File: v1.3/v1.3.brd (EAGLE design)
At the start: 100 x 50.2 mm, 88 parts, among them IC1 LM1117-33, IC2 ENC28J60, K2 G5V1, K3 JRC-21F(4100), T1 2N2222, T2 2N2222, T3 2N2222, T4 2N2222, U1 ATMEGA328P, X1 32.768kHz, X10 22-23-2031, X12 12MHZ, X2 16MHz, X3 25MHz, X9 22-23-2031

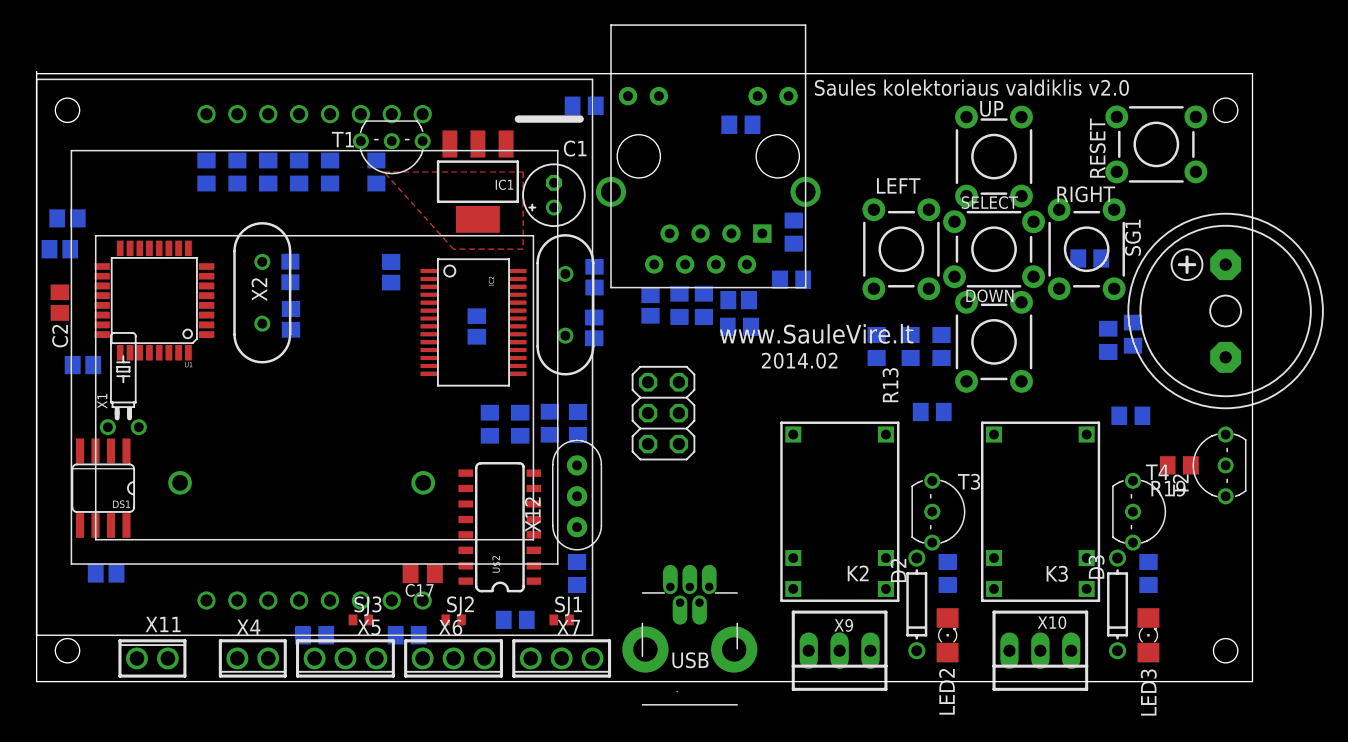
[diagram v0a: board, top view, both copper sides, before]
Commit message: 1.3 versija
programa su 3 klavisais
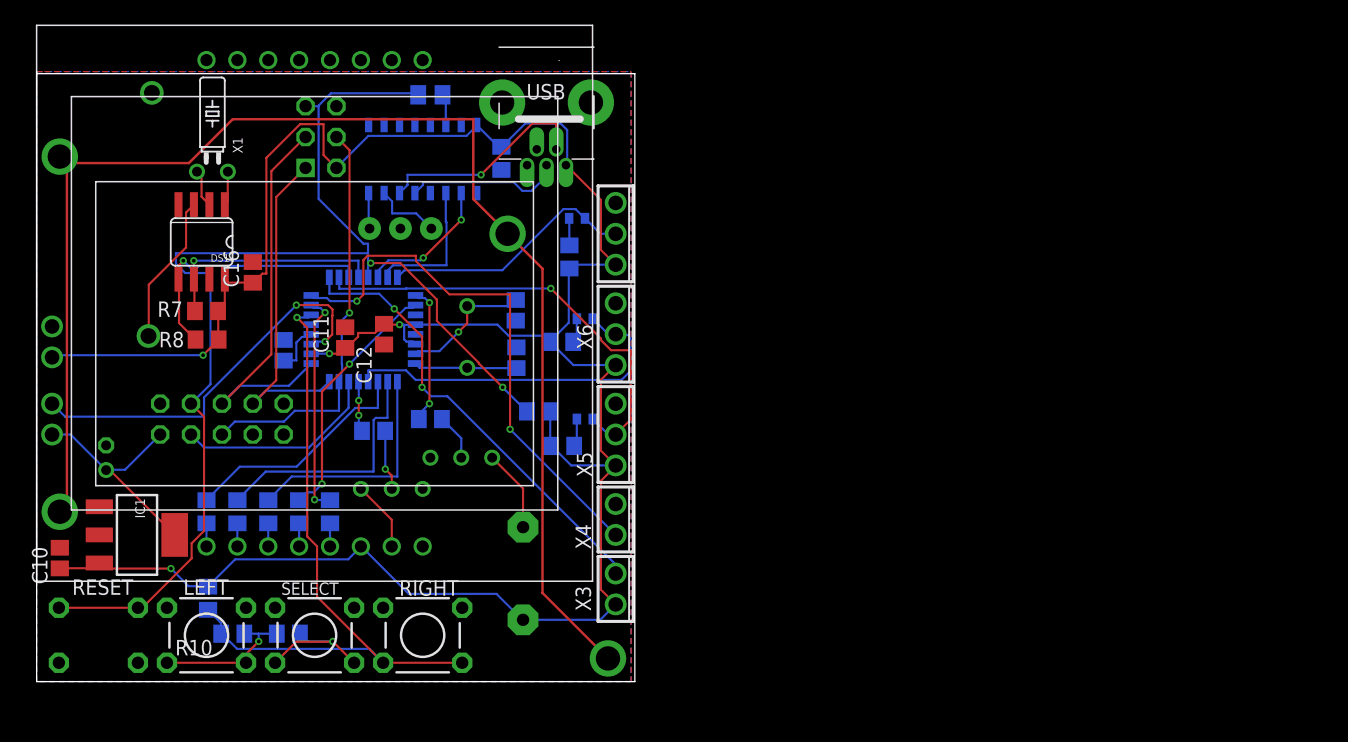
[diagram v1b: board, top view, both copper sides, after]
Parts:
- removed C13: 0.1u, rcl:C0805
- removed C14: 100n, resistor:C0805
- removed C4, C5: 0.1µ, resistor:C0805
- removed C6, C7: 18p, resistor:C0805
- removed CAP: 10u, resistor:C0805
- removed D2, D3: (no value), adafruit:DO-1N4148
- removed DOWN, UP: (no value), SparkFun-Electromechanical:TACTILE-PTH
- removed IC2: ENC28J60, SparkFun-DigitalIC:SSOP28DB
- removed K2: G5V1, relay:G5V1
- removed K3: JRC-21F(4100), relay:G5V1
- removed L1: Bead, rcl:R0805
- removed LED2, LED3: (no value), adafruit:1206
- removed R15, R16, R20: 49, rcl:R0805
- removed R17, R22, R23, R24, R25, R26: 10k, rcl:R0805
- removed R18: 4k7, rcl:R0805
- removed R21: 1k, rcl:R0805
- removed RBS: 2.32K, rcl:R0805
- removed REA, REB: 330, rcl:R0805
- removed RJ1: HR911105A, CONNECTER:HR911105A
- removed T3, T4: 2N2222, adafruit:TO92-EBC-OVAL
- removed X10, X9: 22-23-2031, con-molex:22-23-2031
- removed X12: 12MHZ, adafruit:CERM_OSC
- added ENC28J60: (no value), pinhead:2X05
- added R116: 10k, rcl:R0805
- added X8: (no value), con-phoenix-254:2POL254
- added Y1: 12mhz, SparkFun-FreqCtrl:RESONATOR-PTH
- BAT1, LEFT, RIGHT, SELECT, USB, X11, X4, X5, X6, X7: value (none) -> (none)
- C17: value (none) -> 0.1uF
- ISP: value (none) -> isp
- R1, R3: value 470 -> 10k
- R10: value 330 -> 2k
- R12: value 620 -> 4k7
- R13: value 1k -> 4k7
- R14: value 49 -> 4k7
- R2, R4: value 3k3 -> 10k
- R5: value 4k7 -> 10k
- R6: value 4k7 -> 1k
- SJ1, SJ2, SJ3: value 0R -> (none)
- X3: value 25MHz -> (none); device SparkFun:HC49US -> con-phoenix-254:2POL254
- moved RESET 95.9 mm to (5.08, 3.81), flipped to the bottom, turned to 180 degrees
- moved R1 77.6 mm to (14.0, 14.0), turned to 270 degrees
- moved R9 77.0 mm to (14.1, 6.86), turned to 90 degrees
- moved R10 76.9 mm to (16.1, 3.94), turned to 0 degrees
- moved R2 73.9 mm to (16.5, 14.0), turned to 270 degrees
- moved LEFT 65.4 mm to (14.0, 3.81), turned to 0 degrees
- moved SELECT 64.3 mm to (22.9, 3.81)
- moved RIGHT 63.2 mm to (31.8, 3.81), turned to 0 degrees
- moved R19 61.7 mm to (32.4, 21.6), flipped to the bottom, turned to 0 degrees
- moved SG1 61.7 mm to (40.0, 8.89), flipped to the bottom, turned to 270 degrees
- moved T2 61.6 mm to (34.9, 17.1), flipped to the bottom, turned to 180 degrees
- moved R11 58.7 mm to (20.7, 3.94), turned to 0 degrees
- moved R3 56.1 mm to (19.1, 14.0), turned to 270 degrees
- moved USB 55.4 mm to (41.9, 52.2), turned to 180 degrees
- moved R4 52.7 mm to (21.6, 14.0), turned to 270 degrees
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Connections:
- net N$35 renamed AREF
- net TXD renamed D1/TXD
- removed net D11: IC2.7, ISP.4, U1.15
- removed net D12: IC2.6, ISP.1, U1.16
- removed net D13: IC2.8, U1.17
- removed net LEDA: REA.2, RJ1.G+
- removed net LEDB: REB.2, RJ1.Y+
- removed net N$12: D3.A, K3.9, R1.2, T4.C
- removed net N$13: R2.1, T4.B
- removed net N$14: K2.1, X9.1
- removed net N$16: K3.10, X10.2
- removed net N$19: K3.5, K3.6, X10.3
- removed net N$20: K3.1, X10.1
- removed net N$21: LED3.C, R1.1
- removed net N$22: R22.1, U$1.P$5
- removed net N$23: R25.1, U$1.P$2
- removed net N$24: R24.1, U$1.P$3
- removed net N$25: R23.1, U$1.P$4
- removed net N$34: IC2.27, REA.1
- removed net N$37: IC2.26, REB.1
- removed net N$38: U$2.8, X12.P$3
- removed net N$39: CAP.1, IC2.1
- removed net N$41: C6.1, IC2.24, X3.2
- removed net N$42: C7.1, IC2.23, X3.1
- removed net N$46: R17.1, RESET.3, RESET.4, U1.29
- removed net N$54: C5.2, R15.1, R16.2
- removed net N$59: IC2.14, RBS.2
- removed net N$7 (its old number): LED2.C, R3.1
- removed net N$9: R10.1, R12.2, UP.3, UP.4
- removed net RD+: IC2.13, R15.2, RJ1.RD+
- removed net RD-: IC2.12, R16.1, RJ1.RD-
- removed net RXD: U1.30
- removed net SCK: ISP.3
- removed net SCL: DS1.6, R7.1, U1.28, X4.1
- removed net SDA: DS1.5, R8.1, U1.27, X4.2
- removed net TCT: C4.2, L1.1, R14.2, R20.1, RJ1.P4
- removed net TD+: IC2.17, R20.2, RJ1.TD+
- removed net TD-: IC2.16, R14.1, RJ1.TD-
- removed net V$: R26.1, U$1.P$1
- removed net VIN: ISP.2
- new net A4/SDA: DS1.5, R8.1, U1.27
- new net A5/SCL: DS1.6, R7.1, U1.28
- new net D0/RXD: U$2.2, U1.30
- new net D11/MOSI: ENC28J60.5, ISP.4, U1.15
- new net D12/MISO: ENC28J60.4, ISP.1, U1.16
- new net D13/SCK: ENC28J60.6, ISP.3, U1.17
- net +3V3: now also ENC28J60.9, X8.2; no longer C14.1, IC2.15, IC2.19, IC2.20, IC2.25, IC2.28
- net +5V: now also ISP.2, R116.2, R12.1, R13.1, R14.1, U$1.P$14, X3.2; no longer D2.C, D3.C, K2.2, K3.2, L1.2, LED2.A, LED3.A, R17.2, R18.1, R5.1, R6.1, U$1.P$6
- net A0: now also R5.1; no longer SJ3.2, X5.2
- net A1: now also X4.2; no longer SJ2.2, X6.2
- net A2: now also X3.1; no longer R2.2
- net A3: now also SJ3.2, X5.2; no longer R4.2
- net A6: now also X8.1; no longer R10.2, R9.1, RIGHT.3, RIGHT.4
- net A7: now also R10.2, R9.1, RIGHT.3, RIGHT.4
- net D10: now also ENC28J60.7; no longer R21.2
- net D3: now also R19.2; no longer R22.2
- net D4: now also R4.1; no longer R23.2
- net D5: now also R3.1; no longer R24.2
- net D6: now also R2.1; no longer R25.2
- net D7: now also R1.1; no longer R26.2
- net D8: now also SJ2.2, X6.2; no longer IC2.9
- net D9: now also R6.2; no longer R19.2
- net GND: now also ENC28J60.10, U$1.P$16, X4.1, Y1.2; no longer C13.1, C14.2, C4.1, C5.1, C6.2, C7.2, CAP.2, DOWN.1, DOWN.2, IC2.11, IC2.18, IC2.2, IC2.21, IC2.22, RBS.1, RJ1.G-, RJ1.GND, RJ1.SHIELD0, RJ1.SHIELD1, RJ1.Y-, T3.E, T4.E, U$1.P$8, UP.1, UP.2, X12.P$2
- net N$1: now also R10.1; no longer R13.1
- net N$10: now also Y1.1; no longer X12.P$1
- net N$17: now also R13.2; no longer R6.2
- net N$2: now also R5.2, U$1.P$13; no longer D2.A, K2.9, R3.2, T3.C
- net N$26: now also U$1.P$15; no longer U$1.P$7
- net N$28: now also R14.2; no longer R18.2
- net N$3: now also R4.2, U$1.P$12; no longer R4.1, T3.B
- net N$31: now also R12.2; no longer R5.2
- net N$4: now also R3.2, U$1.P$11; no longer K2.5, K2.6, X9.3
- net N$40: now also U$2.8, Y1.3; no longer C13.2, U$2.4
- net N$44: now also R6.1; no longer R21.1
- net N$5: now also R2.2, U$1.P$10; no longer K2.10, X9.2
- net N$6: now also R1.2, U$1.P$9; no longer DOWN.3, DOWN.4, R12.1, R13.2
- net RESET: now also ENC28J60.8, R116.1, RESET.3, RESET.4, U1.29; no longer IC2.10
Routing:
- net +5V: track 0.00 -> 201.9 mm, vias 0 -> 4
- net GND: track 0.00 -> 114.4 mm, vias 0 -> 4
- net RESET: track 0.00 -> 102.4 mm, vias 0 -> 2
- net A7: track 0.00 -> 55.8 mm, vias 0 -> 1
- net A1: track 0.00 -> 44.7 mm, vias 0 -> 2
- net A2: track 0.00 -> 37.3 mm, vias 0 -> 2
- net A3: track 0.00 -> 37.0 mm, vias 0 -> 1
- net D11/MOSI: track 0.00 -> 33.8 mm, vias 0 -> 1
- net D13/SCK: track 0.00 -> 33.5 mm
- net A6: track 0.00 -> 32.5 mm, vias 0 -> 2
- net D8: track 0.00 -> 29.8 mm
- net D12/MISO: track 0.00 -> 28.2 mm
- net A4/SDA: track 0.00 -> 22.1 mm, vias 0 -> 1
- net D2: track 0.00 -> 21.1 mm
- net D4: track 0.00 -> 20.7 mm, vias 0 -> 2
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- added copper zone on layer 1, net GND
- added copper zone on layer 16, net GND
- removed copper zone on layer 1, net +3V3
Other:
- board size 100 x 50.2 mm -> 49.2 x 50.2 mm
- board text removed: "2014.02"
- board text removed: "Saules kolektoriaus valdiklis v2.0"
- board text removed: "www.SauleVire.lt"
